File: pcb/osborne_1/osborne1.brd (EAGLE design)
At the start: 40 x 97 mm, 19 parts, among them J2 ATX24RH

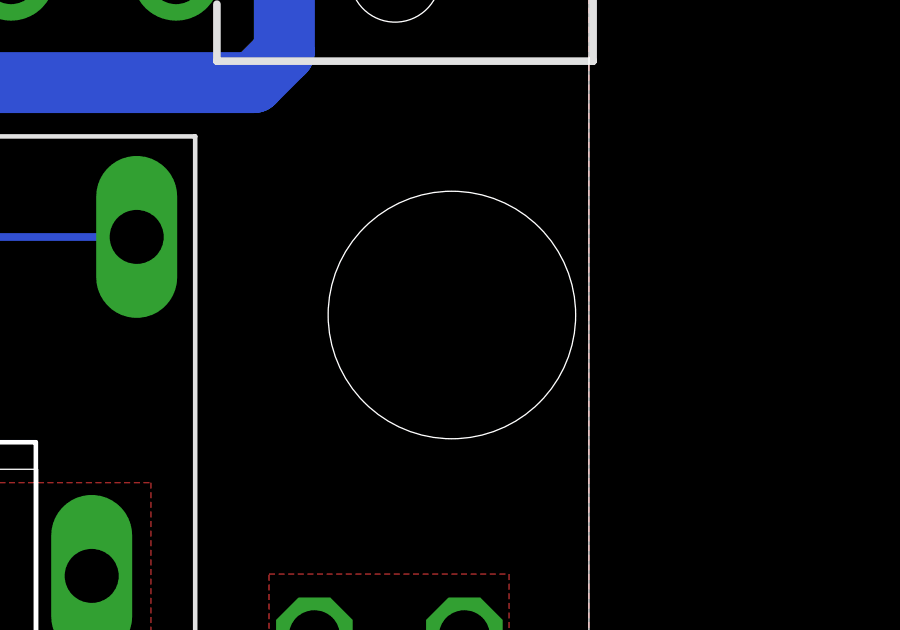
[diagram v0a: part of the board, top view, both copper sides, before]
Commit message: working on new version
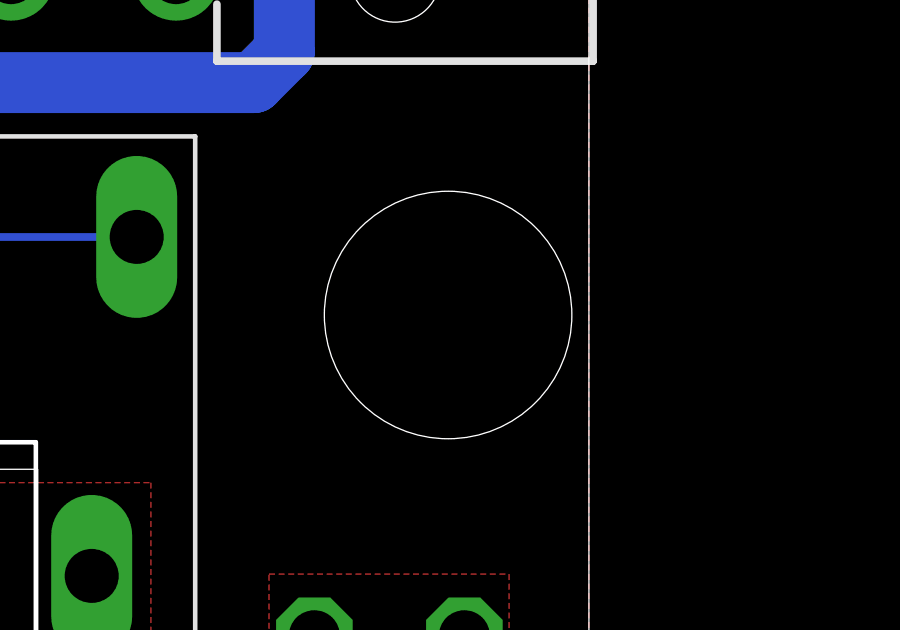
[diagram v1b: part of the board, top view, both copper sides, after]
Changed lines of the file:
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@@
 <text x="8.001" y="5.207" size="2.1844" layer="25" distance="35" align="center">FUSE
 5A MAX</text>
-<hole x="35.433" y="24.13" drill="8.25"/>
+<hole x="35.306" y="24.13" drill="8.25"/>
 <wire x1="45" y1="10" x2="-5" y2="10" width="0.1524" layer="51"/>
 <wire x1="0" y1="87" x2="87" y2="87" width="0.1524" layer="51"/>
